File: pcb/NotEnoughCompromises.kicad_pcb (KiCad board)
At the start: 2 copper layers, 118 parts, among them J1 MJ-4PP-9, J2 MJ-4PP-9, SW1 SW_PUSH, SW10 SW_PUSH, SW11 SW_PUSH, SW12 SW_PUSH, SW13 SW_PUSH, SW14 SW_PUSH, SW15 SW_PUSH, SW16 SW_PUSH, SW17 SW_PUSH, SW18 SW_PUSH, SW19 SW_PUSH, SW2 SW_PUSH, SW20 SW_PUSH, SW21 SW_PUSH, SW22 SW_PUSH, SW23 SW_PUSH, SW24 RESET_SW, SW25 SW_PUSH, SW26 SW_PUSH, SW27 SW_PUSH, SW28 SW_PUSH, SW29 SW_PUSH, SW3 SW_PUSH, SW30 RESET_SW, SW31 SW_PUSH, SW32 SW_PUSH, SW33 SW_PUSH, SW34 SW_PUSH, SW35 SW_PUSH, SW36 SW_PUSH, SW37 SW_PUSH, SW38 SW_PUSH, SW39 SW_PUSH, SW4 SW_PUSH, SW40 SW_PUSH, SW41 SW_PUSH, SW42 SW_PUSH, SW43 SW_PUSH, SW44 SW_PUSH, SW45 SW_PUSH, SW46 SW_PUSH, SW47 SW_PUSH, SW48 SW_PUSH, SW49 SW_PUSH, SW5 SW_PUSH, SW50 SW_PUSH, SW51 SW_PUSH, SW52 SW_PUSH, SW53 SW_PUSH, SW54 SW_PUSH, SW55 SW_PUSH, SW56 SW_PUSH, SW57 SW_PUSH, SW58 SW_PUSH, SW6 SW_PUSH, SW7 SW_PUSH, SW8 SW_PUSH, SW9 SW_PUSH, U1 ProMicro, U2 ProMicro

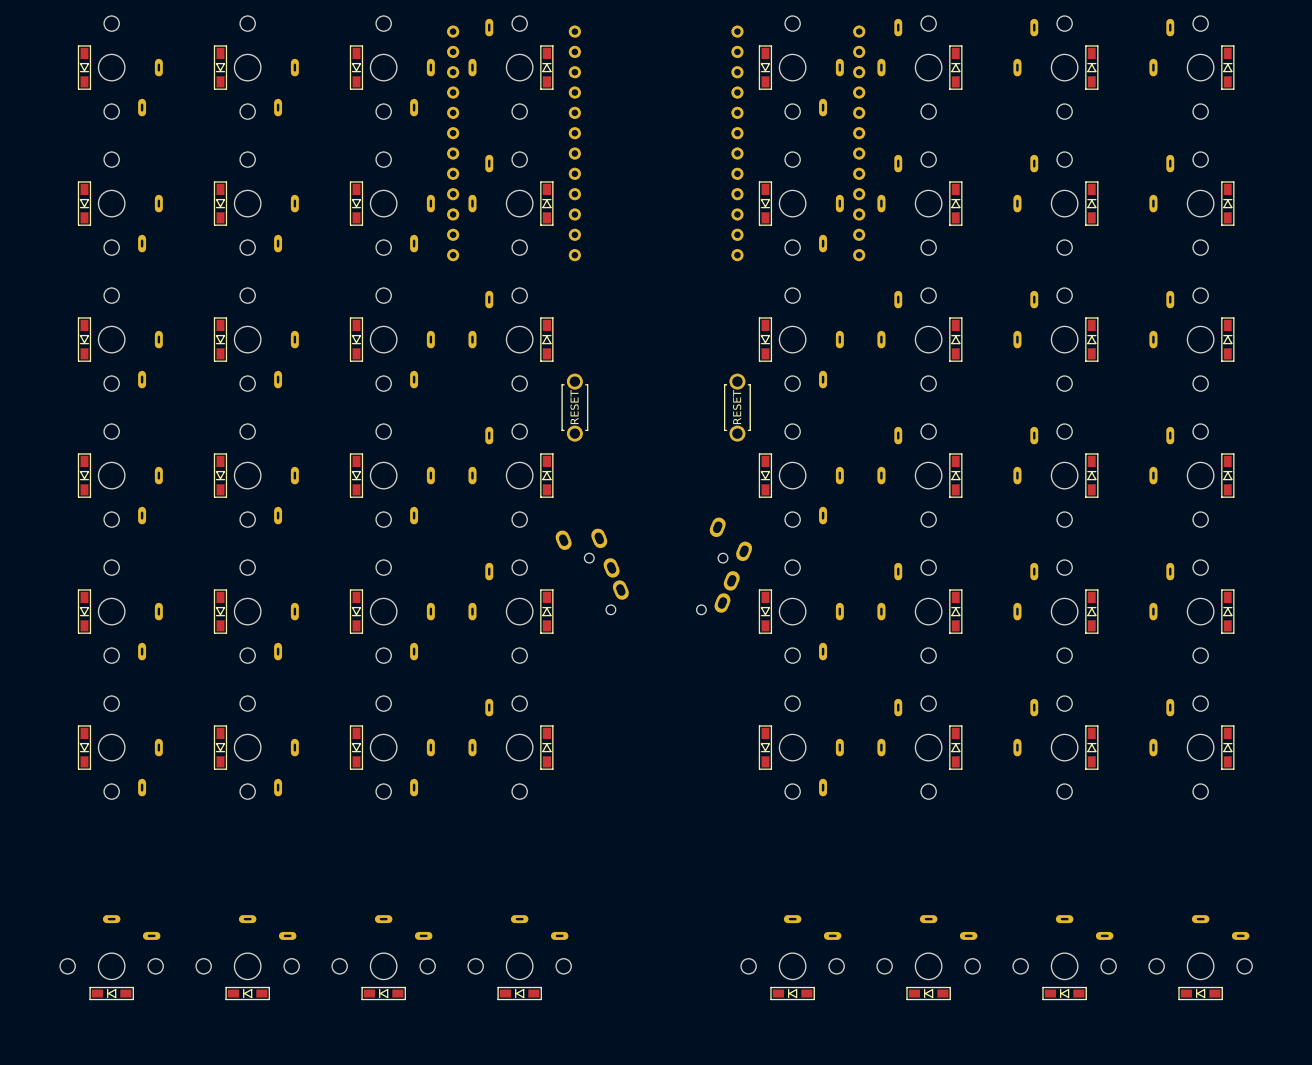
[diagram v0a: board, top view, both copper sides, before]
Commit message: 基板を作成
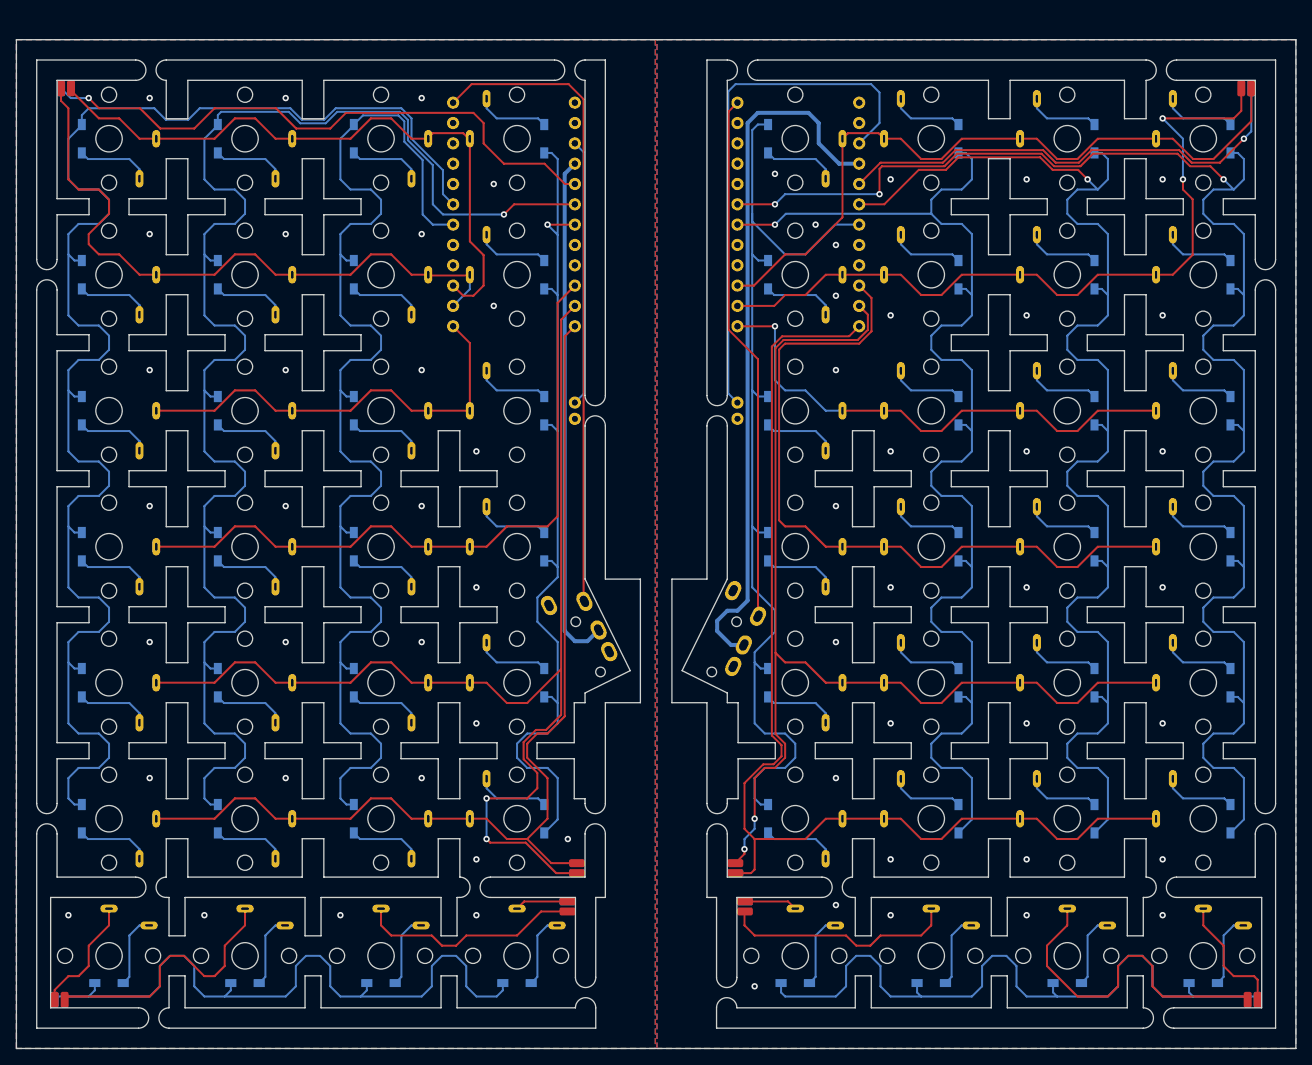
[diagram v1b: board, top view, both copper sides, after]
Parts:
- added J1: Conn_01x01_Socket, Connector_Wire:SolderWirePad_1x01_SMD_1x2mm, B.Cu at (137.4, 133.1)
- added J10: Conn_01x01_Pin, Connector_Wire:SolderWirePad_1x01_SMD_1x2mm, F.Cu at (136.2, 137.9)
- added J12: Conn_01x01_Socket, Connector_Wire:SolderWirePad_1x01_SMD_1x2mm, F.Cu at (137.4, 133.1)
- added J13: Conn_01x01_Pin, Connector_Wire:SolderWirePad_1x01_SMD_1x2mm, F.Cu at (136.2, 136.7)
- added J14: Conn_01x01_Socket, Connector_Wire:SolderWirePad_1x01_SMD_1x2mm, B.Cu at (221.7, 35.0)
- added J15: Conn_01x01_Pin, Connector_Wire:SolderWirePad_1x01_SMD_1x2mm, B.Cu at (222.5, 149.0)
- added J17: Conn_01x01_Socket, Connector_Wire:SolderWirePad_1x01_SMD_1x2mm, F.Cu at (157.2, 133.1)
- added J18: Conn_01x01_Pin, Connector_Wire:SolderWirePad_1x01_SMD_1x2mm, F.Cu at (158.4, 136.7)
- added J19: Conn_01x01_Socket, Connector_Wire:SolderWirePad_1x01_SMD_1x2mm, F.Cu at (157.2, 131.9)
- added J2: Conn_01x01_Socket, Connector_Wire:SolderWirePad_1x01_SMD_1x2mm, B.Cu at (72.9, 35.0)
- added J20: Conn_01x01_Pin, Connector_Wire:SolderWirePad_1x01_SMD_1x2mm, F.Cu at (158.4, 137.9)
- added J21: Conn_01x01_Socket, Connector_Wire:SolderWirePad_1x01_SMD_1x2mm, F.Cu at (220.5, 35.0)
- added J22: Conn_01x01_Pin, Connector_Wire:SolderWirePad_1x01_SMD_1x2mm, F.Cu at (221.3, 149.0)
- added J23: Conn_01x01_Socket, Connector_Wire:SolderWirePad_1x01_SMD_1x2mm, F.Cu at (221.7, 35.0)
- added J24: Conn_01x01_Pin, Connector_Wire:SolderWirePad_1x01_SMD_1x2mm, F.Cu at (222.5, 149.0)
- added J25: Conn_01x01_Socket, Connector_Wire:SolderWirePad_1x01_SMD_1x2mm, B.Cu at (157.2, 133.1)
- added J26: Conn_01x01_Pin, Connector_Wire:SolderWirePad_1x01_SMD_1x2mm, B.Cu at (158.4, 136.7)
- added J3: Conn_01x01_Pin, Connector_Wire:SolderWirePad_1x01_SMD_1x2mm, B.Cu at (136.2, 136.7)
- added J4: Conn_01x01_Pin, Connector_Wire:SolderWirePad_1x01_SMD_1x2mm, B.Cu at (72.1, 149.0)
- added J5: Conn_01x01_Socket, Connector_Wire:SolderWirePad_1x01_SMD_1x2mm, F.Cu at (72.9, 35.0)
- added J6: Conn_01x01_Pin, Connector_Wire:SolderWirePad_1x01_SMD_1x2mm, F.Cu at (72.1, 149.0)
- added J7: Conn_01x01_Socket, Connector_Wire:SolderWirePad_1x01_SMD_1x2mm, F.Cu at (74.2, 35.0)
- added J8: Conn_01x01_Pin, Connector_Wire:SolderWirePad_1x01_SMD_1x2mm, F.Cu at (73.4, 149.0)
- added J9: Conn_01x01_Socket, Connector_Wire:SolderWirePad_1x01_SMD_1x2mm, F.Cu at (137.4, 131.9)
- D1, D10, D11, D12, D13, D14, D15, D16, D17, D18, D19, D2, D20, D21, D22, D23, D24, D25, D26, D27, D28, D29, D3, D30, D31, D32, D33, D34, D35, D36, D37, D38, D39, D4, D40, D41, D42, D43, D44, D45, D46, D47, D48, D49, D5, D50, D51, D52, D53, D54, D55, D56, D6, D7, D8, D9: moved to B.Cu
- SW24, SW30: footprint kbd:ResetSW_1side -> not_enough_compromises:reset_sw
- moved D1 8.90 mm to (133.3, 41.3), turned to 90 degrees
- moved D10 8.90 mm to (109.5, 75.3), turned to -90 degrees
- moved D11 8.90 mm to (92.5, 75.3), turned to -90 degrees
- moved D12 8.90 mm to (75.5, 75.3), turned to -90 degrees
- moved D14 8.90 mm to (133.3, 92.3), turned to 90 degrees
- moved D15 8.90 mm to (109.5, 92.3), turned to -90 degrees
- moved D16 8.90 mm to (92.5, 92.3), turned to -90 degrees
- moved D17 8.90 mm to (75.5, 92.3), turned to -90 degrees
- moved D19 8.90 mm to (133.3, 109.3), turned to 90 degrees
- moved D2 8.90 mm to (109.5, 41.3), turned to -90 degrees
- moved D20 8.90 mm to (109.5, 109.3), turned to -90 degrees
- moved D21 8.90 mm to (92.5, 109.3), turned to -90 degrees
- moved D22 8.90 mm to (75.5, 109.3), turned to -90 degrees
- moved D24 8.90 mm to (133.3, 126.3), turned to 90 degrees
- moved D25 8.90 mm to (109.5, 126.3), turned to -90 degrees
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- renumbered J1 to J11, J2 to J16
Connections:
- D1 pad 2: Net-(D1-Pad2) -> Net-(D1-A)
- D10 pad 2: Net-(D10-Pad2) -> Net-(D10-A)
- D11 pad 2: Net-(D11-Pad2) -> Net-(D11-A)
- D12 pad 2: Net-(D12-Pad2) -> Net-(D12-A)
- D13 pad 1: l_row4 -> Net-(D13-K)
- D13 pad 2: Net-(D13-Pad2) -> Net-(D13-A)
- D14 pad 2: Net-(D14-Pad2) -> Net-(D14-A)
- D15 pad 2: Net-(D15-Pad2) -> Net-(D15-A)
- D16 pad 2: Net-(D16-Pad2) -> Net-(D16-A)
- D17 pad 2: Net-(D17-Pad2) -> Net-(D17-A)
- D18 pad 1: l_row4 -> Net-(D13-K)
- D18 pad 2: Net-(D18-Pad2) -> Net-(D18-A)
- D19 pad 2: Net-(D19-Pad2) -> Net-(D19-A)
- D2 pad 2: Net-(D2-Pad2) -> Net-(D2-A)
- D20 pad 2: Net-(D20-Pad2) -> Net-(D20-A)
- D21 pad 2: Net-(D21-Pad2) -> Net-(D21-A)
- D22 pad 2: Net-(D22-Pad2) -> Net-(D22-A)
- D23 pad 1: l_row4 -> Net-(D13-K)
- D23 pad 2: Net-(D23-Pad2) -> Net-(D23-A)
- D24 pad 2: Net-(D24-Pad2) -> Net-(D24-A)
- D25 pad 2: Net-(D25-Pad2) -> Net-(D25-A)
- D26 pad 2: Net-(D26-Pad2) -> Net-(D26-A)
- D27 pad 2: Net-(D27-Pad2) -> Net-(D27-A)
- D28 pad 1: l_row4 -> Net-(D13-K)
- D28 pad 2: Net-(D28-Pad2) -> Net-(D28-A)
- D29 pad 2: Net-(D29-Pad2) -> Net-(D29-A)
- D3 pad 2: Net-(D3-Pad2) -> Net-(D3-A)
- D30 pad 2: Net-(D30-Pad2) -> Net-(D30-A)
- D31 pad 2: Net-(D31-Pad2) -> Net-(D31-A)
- D32 pad 2: Net-(D32-Pad2) -> Net-(D32-A)
- D33 pad 1: r_row4 -> Net-(D33-K)
- D33 pad 2: Net-(D33-Pad2) -> Net-(D33-A)
- D34 pad 2: Net-(D34-Pad2) -> Net-(D34-A)
- D35 pad 2: Net-(D35-Pad2) -> Net-(D35-A)
- D36 pad 2: Net-(D36-Pad2) -> Net-(D36-A)
- D37 pad 2: Net-(D37-Pad2) -> Net-(D37-A)
- D38 pad 1: r_row4 -> Net-(D33-K)
- D38 pad 2: Net-(D38-Pad2) -> Net-(D38-A)
- D39 pad 2: Net-(D39-Pad2) -> Net-(D39-A)
- D4 pad 2: Net-(D4-Pad2) -> Net-(D4-A)
- D40 pad 2: Net-(D40-Pad2) -> Net-(D40-A)
- D41 pad 2: Net-(D41-Pad2) -> Net-(D41-A)
- D42 pad 2: Net-(D42-Pad2) -> Net-(D42-A)
- D43 pad 1: r_row4 -> Net-(D33-K)
- D43 pad 2: Net-(D43-Pad2) -> Net-(D43-A)
- D44 pad 2: Net-(D44-Pad2) -> Net-(D44-A)
- D45 pad 2: Net-(D45-Pad2) -> Net-(D45-A)
- D46 pad 2: Net-(D46-Pad2) -> Net-(D46-A)
- D47 pad 2: Net-(D47-Pad2) -> Net-(D47-A)
- D48 pad 1: r_row4 -> Net-(D33-K)
- D48 pad 2: Net-(D48-Pad2) -> Net-(D48-A)
- D49 pad 2: Net-(D49-Pad2) -> Net-(D49-A)
- D5 pad 2: Net-(D5-Pad2) -> Net-(D5-A)
- D50 pad 2: Net-(D50-Pad2) -> Net-(D50-A)
- D51 pad 2: Net-(D51-Pad2) -> Net-(D51-A)
- D52 pad 2: Net-(D52-Pad2) -> Net-(D52-A)
- D53 pad 2: Net-(D53-Pad2) -> Net-(D53-A)
- D54 pad 2: Net-(D54-Pad2) -> Net-(D54-A)
- D55 pad 2: Net-(D55-Pad2) -> Net-(D55-A)
- D56 pad 2: Net-(D56-Pad2) -> Net-(D56-A)
- D6 pad 2: Net-(D6-Pad2) -> Net-(D6-A)
- D7 pad 2: Net-(D7-Pad2) -> Net-(D7-A)
- D8 pad 2: Net-(D8-Pad2) -> Net-(D8-A)
- D9 pad 2: Net-(D9-Pad2) -> Net-(D9-A)
- SW1 pad 1: l_col0 -> Net-(D1-A)
- SW1 pad 2: Net-(D1-Pad2) -> l_col0
- SW10 pad 1: l_col2 -> Net-(D10-A)
- SW10 pad 2: Net-(D10-Pad2) -> l_col2
- SW11 pad 1: l_col2 -> Net-(D11-A)
- SW11 pad 2: Net-(D11-Pad2) -> l_col2
- SW12 pad 1: l_col2 -> Net-(D12-A)
- SW12 pad 2: Net-(D12-Pad2) -> l_col2
- SW13 pad 1: l_col0 -> Net-(D13-A)
- SW13 pad 2: Net-(D13-Pad2) -> Net-(J6-Pin_1)
- SW14 pad 1: l_col3 -> Net-(D14-A)
- SW14 pad 2: Net-(D14-Pad2) -> l_col3
- SW15 pad 1: l_col3 -> Net-(D15-A)
- SW15 pad 2: Net-(D15-Pad2) -> l_col3
- SW16 pad 1: l_col3 -> Net-(D16-A)
- SW16 pad 2: Net-(D16-Pad2) -> l_col3
- SW17 pad 1: l_col3 -> Net-(D17-A)
- SW17 pad 2: Net-(D17-Pad2) -> l_col3
- SW18 pad 1: l_col1 -> Net-(D18-A)
- SW18 pad 2: Net-(D18-Pad2) -> Net-(J8-Pin_1)
- SW19 pad 1: l_col4 -> Net-(D19-A)
- SW19 pad 2: Net-(D19-Pad2) -> l_col4
- SW2 pad 1: l_col0 -> Net-(D2-A)
- SW2 pad 2: Net-(D2-Pad2) -> l_col0
- SW20 pad 1: l_col4 -> Net-(D20-A)
- SW20 pad 2: Net-(D20-Pad2) -> l_col4
- SW21 pad 1: l_col4 -> Net-(D21-A)
- SW21 pad 2: Net-(D21-Pad2) -> l_col4
- SW22 pad 1: l_col4 -> Net-(D22-A)
- SW22 pad 2: Net-(D22-Pad2) -> l_col4
- SW23 pad 1: l_col4 -> Net-(D23-A)
- SW23 pad 2: Net-(D23-Pad2) -> Net-(J10-Pin_1)
- SW25 pad 1: l_col5 -> Net-(D24-A)
- SW25 pad 2: Net-(D24-Pad2) -> l_col5
- SW26 pad 1: l_col5 -> Net-(D25-A)
- SW26 pad 2: Net-(D25-Pad2) -> l_col5
- SW27 pad 1: l_col5 -> Net-(D26-A)
- SW27 pad 2: Net-(D26-Pad2) -> l_col5
- SW28 pad 1: l_col5 -> Net-(D27-A)
- SW28 pad 2: Net-(D27-Pad2) -> l_col5
- SW29 pad 1: l_col5 -> Net-(D28-A)
- SW29 pad 2: Net-(D28-Pad2) -> Net-(J13-Pin_1)
- SW3 pad 1: l_col0 -> Net-(D3-A)
- SW3 pad 2: Net-(D3-Pad2) -> l_col0
- SW31 pad 1: r_col5 -> Net-(D29-A)
- SW31 pad 2: Net-(D29-Pad2) -> r_col5
- SW32 pad 1: r_col5 -> Net-(D30-A)
- SW32 pad 2: Net-(D30-Pad2) -> r_col5
- SW33 pad 1: r_col5 -> Net-(D31-A)
- SW33 pad 2: Net-(D31-Pad2) -> r_col5
- SW34 pad 1: r_col5 -> Net-(D32-A)
- SW34 pad 2: Net-(D32-Pad2) -> r_col5
- SW35 pad 1: r_col5 -> Net-(D33-A)
- SW35 pad 2: Net-(D33-Pad2) -> Net-(J18-Pin_1)
- SW36 pad 1: r_col4 -> Net-(D34-A)
- SW36 pad 2: Net-(D34-Pad2) -> r_col4
- SW37 pad 1: r_col4 -> Net-(D35-A)
- SW37 pad 2: Net-(D35-Pad2) -> r_col4
- SW38 pad 1: r_col4 -> Net-(D36-A)
- SW38 pad 2: Net-(D36-Pad2) -> r_col4
- SW39 pad 1: r_col4 -> Net-(D37-A)
- SW39 pad 2: Net-(D37-Pad2) -> r_col4
- SW4 pad 1: l_col0 -> Net-(D4-A)
- SW4 pad 2: Net-(D4-Pad2) -> l_col0
- SW40 pad 1: r_col4 -> Net-(D38-A)
- SW40 pad 2: Net-(D38-Pad2) -> Net-(J20-Pin_1)
- SW41 pad 1: r_col3 -> Net-(D39-A)
- SW41 pad 2: Net-(D39-Pad2) -> r_col3
- SW42 pad 1: r_col3 -> Net-(D40-A)
- SW42 pad 2: Net-(D40-Pad2) -> r_col3
- SW43 pad 1: r_col3 -> Net-(D41-A)
- SW43 pad 2: Net-(D41-Pad2) -> r_col3
- SW44 pad 1: r_col3 -> Net-(D42-A)
- SW44 pad 2: Net-(D42-Pad2) -> r_col3
- SW45 pad 1: r_col1 -> Net-(D43-A)
- SW45 pad 2: Net-(D43-Pad2) -> Net-(J22-Pin_1)
- SW46 pad 1: r_col2 -> Net-(D44-A)
- SW46 pad 2: Net-(D44-Pad2) -> r_col2
- SW47 pad 1: r_col2 -> Net-(D45-A)
- SW47 pad 2: Net-(D45-Pad2) -> r_col2
- SW48 pad 1: r_col2 -> Net-(D46-A)
- SW48 pad 2: Net-(D46-Pad2) -> r_col2
- SW49 pad 1: r_col2 -> Net-(D47-A)
- SW49 pad 2: Net-(D47-Pad2) -> r_col2
- SW5 pad 1: l_col1 -> Net-(D5-A)
- SW5 pad 2: Net-(D5-Pad2) -> l_col1
- SW50 pad 1: r_col0 -> Net-(D48-A)
- SW50 pad 2: Net-(D48-Pad2) -> Net-(J24-Pin_1)
- SW51 pad 1: r_col1 -> Net-(D49-A)
- SW51 pad 2: Net-(D49-Pad2) -> r_col1
- SW52 pad 1: r_col1 -> Net-(D50-A)
- SW52 pad 2: Net-(D50-Pad2) -> r_col1
- SW53 pad 1: r_col1 -> Net-(D51-A)
- SW53 pad 2: Net-(D51-Pad2) -> r_col1
- SW54 pad 1: r_col1 -> Net-(D52-A)
- SW54 pad 2: Net-(D52-Pad2) -> r_col1
- SW55 pad 1: r_col0 -> Net-(D53-A)
- SW55 pad 2: Net-(D53-Pad2) -> r_col0
- SW56 pad 1: r_col0 -> Net-(D54-A)
- SW56 pad 2: Net-(D54-Pad2) -> r_col0
- SW57 pad 1: r_col0 -> Net-(D55-A)
- SW57 pad 2: Net-(D55-Pad2) -> r_col0
- SW58 pad 1: r_col0 -> Net-(D56-A)
- SW58 pad 2: Net-(D56-Pad2) -> r_col0
- SW6 pad 1: l_col1 -> Net-(D6-A)
- SW6 pad 2: Net-(D6-Pad2) -> l_col1
- SW7 pad 1: l_col1 -> Net-(D7-A)
- SW7 pad 2: Net-(D7-Pad2) -> l_col1
- SW8 pad 1: l_col1 -> Net-(D8-A)
- SW8 pad 2: Net-(D8-Pad2) -> l_col1
- SW9 pad 1: l_col2 -> Net-(D9-A)
- SW9 pad 2: Net-(D9-Pad2) -> l_col2
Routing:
- net r_row3: track 0.00 -> 200.5 mm, vias 0 -> 3
- net l_row3: track 0.00 -> 189.4 mm
- net l_row2: track 0.00 -> 188.2 mm, vias 0 -> 1
- net r_row2: track 0.00 -> 164.8 mm, vias 0 -> 1
- net r_row1: track 0.00 -> 155.6 mm, vias 0 -> 1
- net l_row1: track 0.00 -> 154.8 mm
- net l_col4: track 0.00 -> 147.1 mm, vias 0 -> 2
- net r_col5: track 0.00 -> 139.1 mm
- net r_col4: track 0.00 -> 137.5 mm, vias 0 -> 2
- net l_col5: track 0.00 -> 128.5 mm
- net r_row0: track 0.00 -> 123.7 mm
- net l_row0: track 0.00 -> 109.4 mm, vias 0 -> 1
- net r_col1: track 0.00 -> 95.4 mm, vias 0 -> 2
- net r_col3: track 0.00 -> 92.9 mm
- net r_col0: track 0.00 -> 89.5 mm
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- added copper zone on B.Cu, net l_GND
- added copper zone on F.Cu, net l_GND
- added copper zone on B.Cu, net r_GND
- added copper zone on F.Cu, net r_GND
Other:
- board outline added: 159.9 x 126.1 mm
